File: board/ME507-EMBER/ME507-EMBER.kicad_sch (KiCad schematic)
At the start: 6 parts, among them J1 Screw_Terminal_01x02, J2 Screw_Terminal_01x02, J3 Screw_Terminal_01x02, Q1 Q_NMOS_GDS

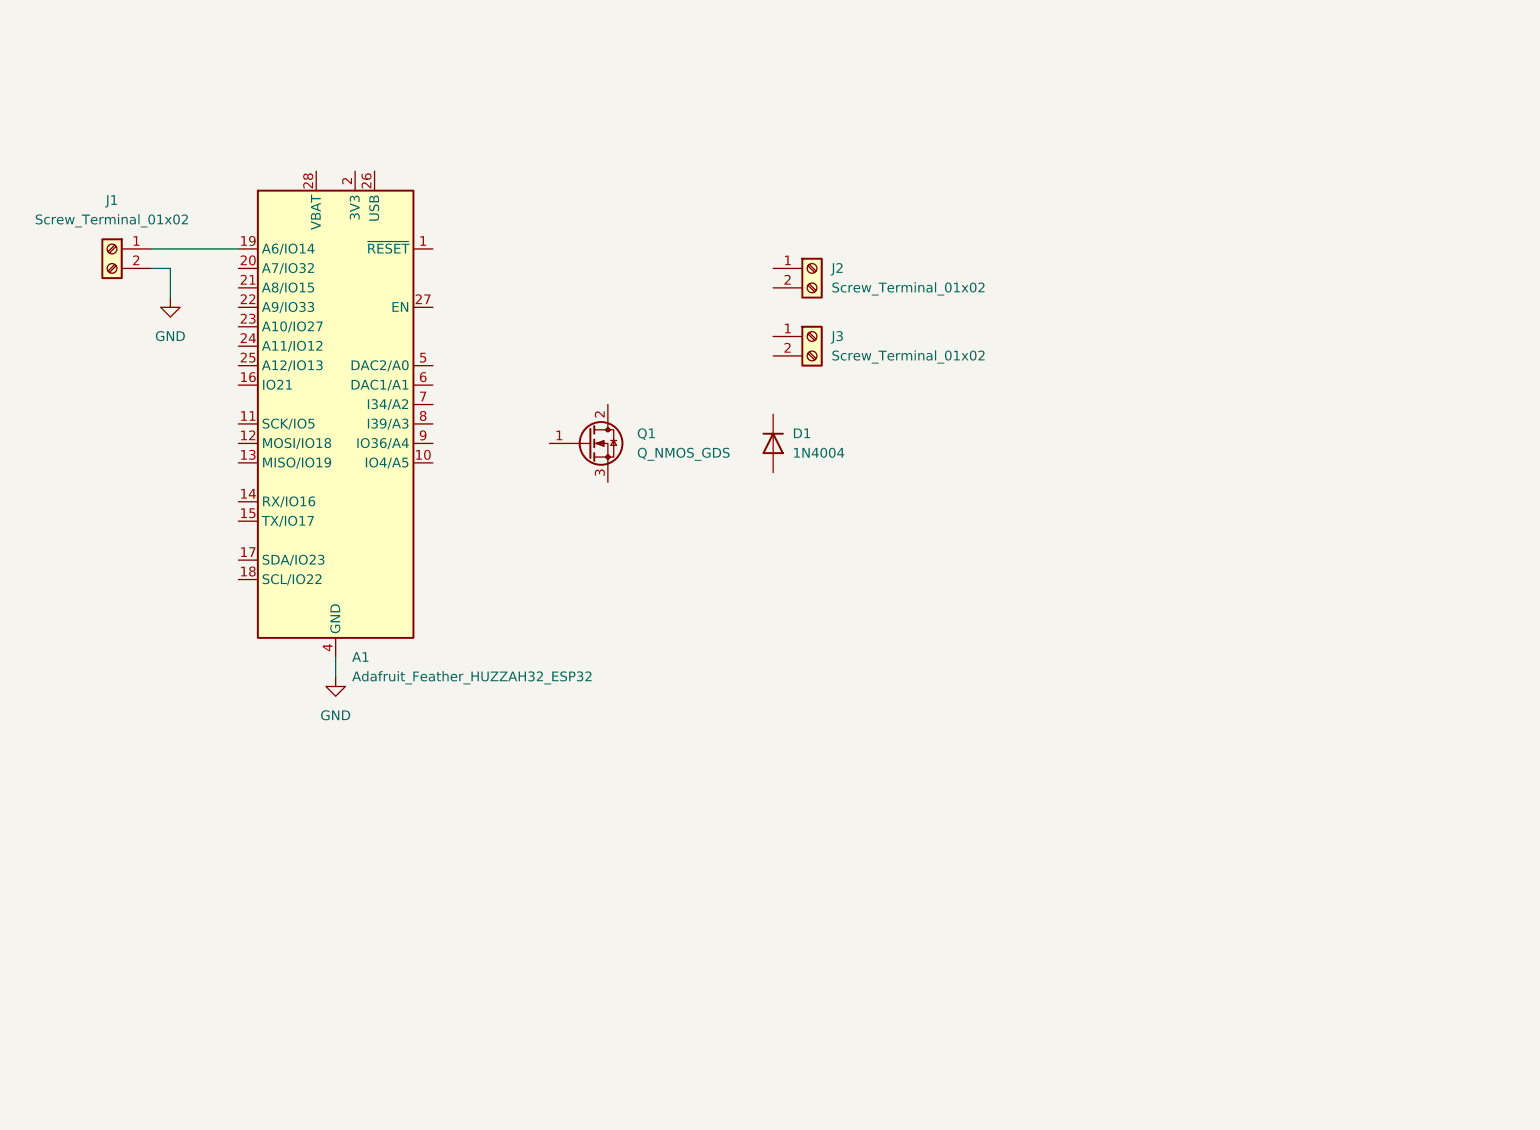
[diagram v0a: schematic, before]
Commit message: modified:   board/ME507-EMBER/ME507-EMBER.kicad_sch 	deleted:    board/ME507-EMBER/~ME507-EMBER.kicad_sch.lck
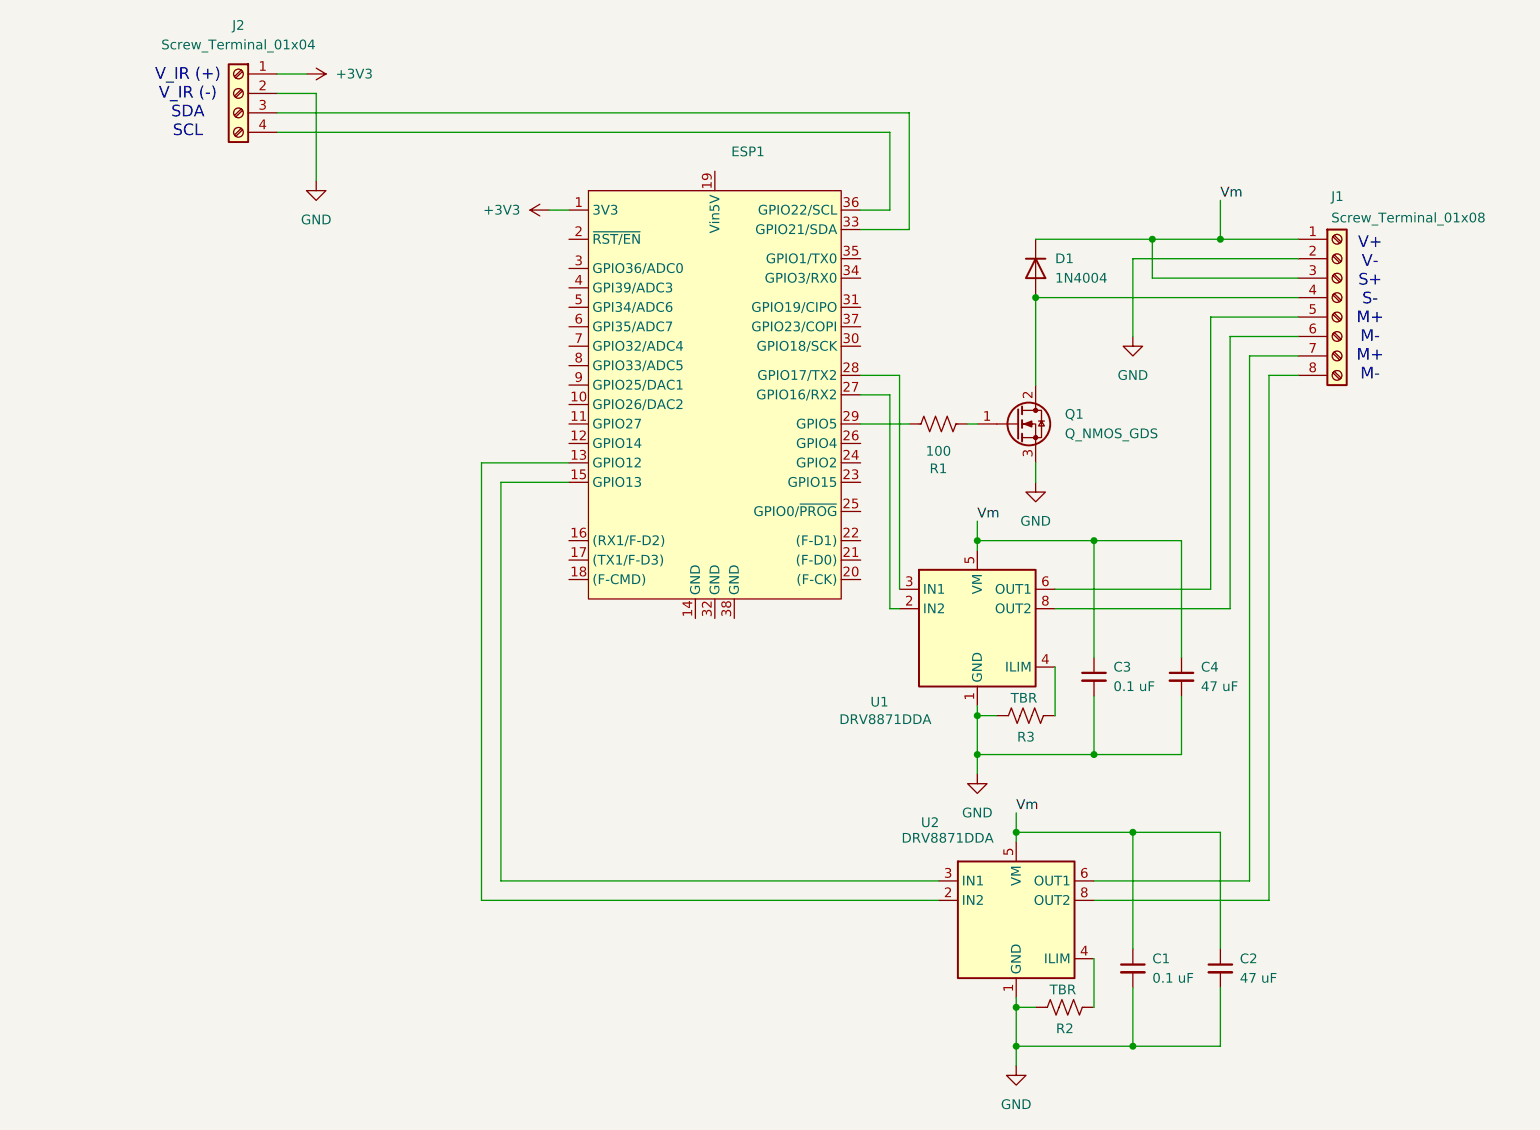
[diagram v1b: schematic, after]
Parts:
- removed A1: Adafruit_Feather_HUZZAH32_ESP32, Module:Adafruit_Feather, symbol MCU_Module:Adafruit_Feather_HUZZAH32_ESP32
- removed J1, J3: Screw_Terminal_01x02, symbol Connector:Screw_Terminal_01x02
- removed J2: Screw_Terminal_01x02, TerminalBlock_4Ucon:TerminalBlock_4Ucon_1x02_P3.50mm_Horizontal, symbol Connector:Screw_Terminal_01x02
- added C1, C3: 0.1 uF, symbol Device:C_Small
- added C2, C4: 47 uF, symbol Device:C_Small
- added ESP1: ~, ME507F24:ESP32_NodeMCU_KeeYees, symbol ME507F24:ESP32_Node_KY
- added J1: Screw_Terminal_01x08, TerminalBlock_Phoenix:TerminalBlock_Phoenix_MPT-0,5-8-2.54_1x08_P2.54mm_Horizontal, symbol Connector:Screw_Terminal_01x08
- added J2: Screw_Terminal_01x04, symbol Connector:Screw_Terminal_01x04
- added R1: 100, symbol Device:R_US
- added R2, R3: TBR, symbol Device:R_US
- added U1, U2: DRV8871DDA, Package_SO:Texas_HTSOP-8-1EP_3.9x4.9mm_P1.27mm_EP2.95x4.9mm_Mask2.4x3.1mm_ThermalVias, symbol Driver_Motor:DRV8871DDA
- Q1: footprint (none) -> Package_TO_SOT_SMD:TSOT-23
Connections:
- net GND: now also Q1.3 (S), C1.2, C2.2, C3.2, C4.2, J1.2 (Pin_2), J2.2 (Pin_2), R2.1, R3.1, U1.1 (GND), U1.7 (GND), U1.9 (GND), U2.1 (GND), U2.7 (GND), U2.9 (GND)
- net Vm: now reaches D1.1 (K)
- net Vm: now also C1.1, C2.1, C3.1, C4.1, J1.1 (Pin_1), J1.3 (Pin_3), U1.5 (VM), U2.5 (VM)
- net at D1.2 (A): now also Q1.2 (D), J1.4 (Pin_4)
- net at Q1.1 (G): now also R1.2
- new net: ESP1.33 (GPIO21/SDA), J2.3 (Pin_3)
- new net: ESP1.36 (GPIO22/SCL), J2.4 (Pin_4)
- new net: ESP1.27 (GPIO16/RX2), U1.2 (IN2)
- new net: ESP1.28 (GPIO17/TX2), U1.3 (IN1)
- new net: R3.2, U1.4 (ILIM)
- new net: J1.5 (Pin_5), U1.6 (OUT1)
- new net: J1.6 (Pin_6), U1.8 (OUT2)
- new net: ESP1.29 (GPIO5), R1.1
- new net: ESP1.13 (GPIO12), U2.2 (IN2)
- new net: ESP1.15 (GPIO13), U2.3 (IN1)
- new net: R2.2, U2.4 (ILIM)
- new net: J1.7 (Pin_7), U2.6 (OUT1)
- new net: J1.8 (Pin_8), U2.8 (OUT2)
- new net +3V3: ESP1.1 (3V3), J2.1 (Pin_1)
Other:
- note added: "V+ V- S+ S- M+ M- M+ M-"
- note added: "V_IR (+) V_IR (-) SDA SCL"
